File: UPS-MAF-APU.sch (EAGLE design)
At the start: 32 parts, among them J1 CONNECTOR_PI_40_PIN, J2 Barrel DC In, J3 OLED, J4 OSTOQ045451, J5 External DS18B20 Temp, J6 FTDI Serial Console, J7 MagJack, U1 OLED_I2C, U2 SI7006-A20-IM, U4 INA260AIPW, U6 ENC28J60_SS, U7 5V SMPS, Y1 ECS-250-20-3X-EN-TR

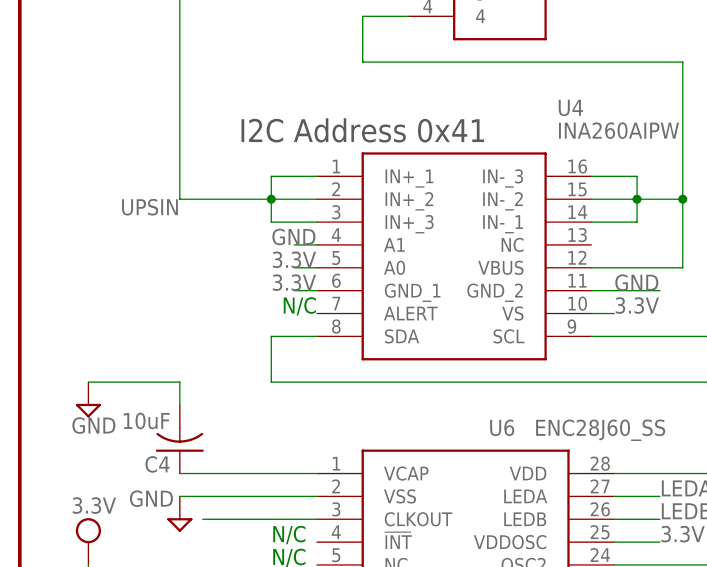
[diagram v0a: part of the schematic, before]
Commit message: README
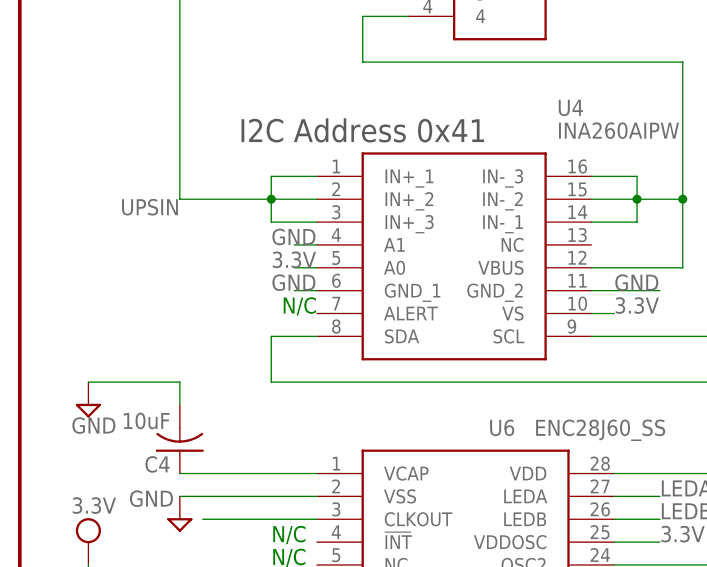
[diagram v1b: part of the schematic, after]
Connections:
- net 3.3V: no longer U4.GND_1
- net GND: now also U4.GND_1
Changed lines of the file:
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@@
 <label x="35.56" y="193.04" size="1.778" layer="95"/>
+</segment>
+<segment>
+<pinref part="U4" gate="G$1" pin="GND_1"/>
+<wire x1="33.02" y1="160.02" x2="30.48" y2="160.02" width="0.1524" layer="91"/>
+<label x="27.94" y="160.02" size="1.778" layer="95"/>
 </segment>
 </net>
@@
 </segment>
 <segment>
-<pinref part="U4" gate="G$1" pin="GND_1"/>
-<wire x1="33.02" y1="160.02" x2="30.48" y2="160.02" width="0.1524" layer="91"/>
-<label x="27.94" y="160.02" size="1.778" layer="95"/>
-</segment>
-<segment>
